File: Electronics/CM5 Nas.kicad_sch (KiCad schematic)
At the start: 0 parts

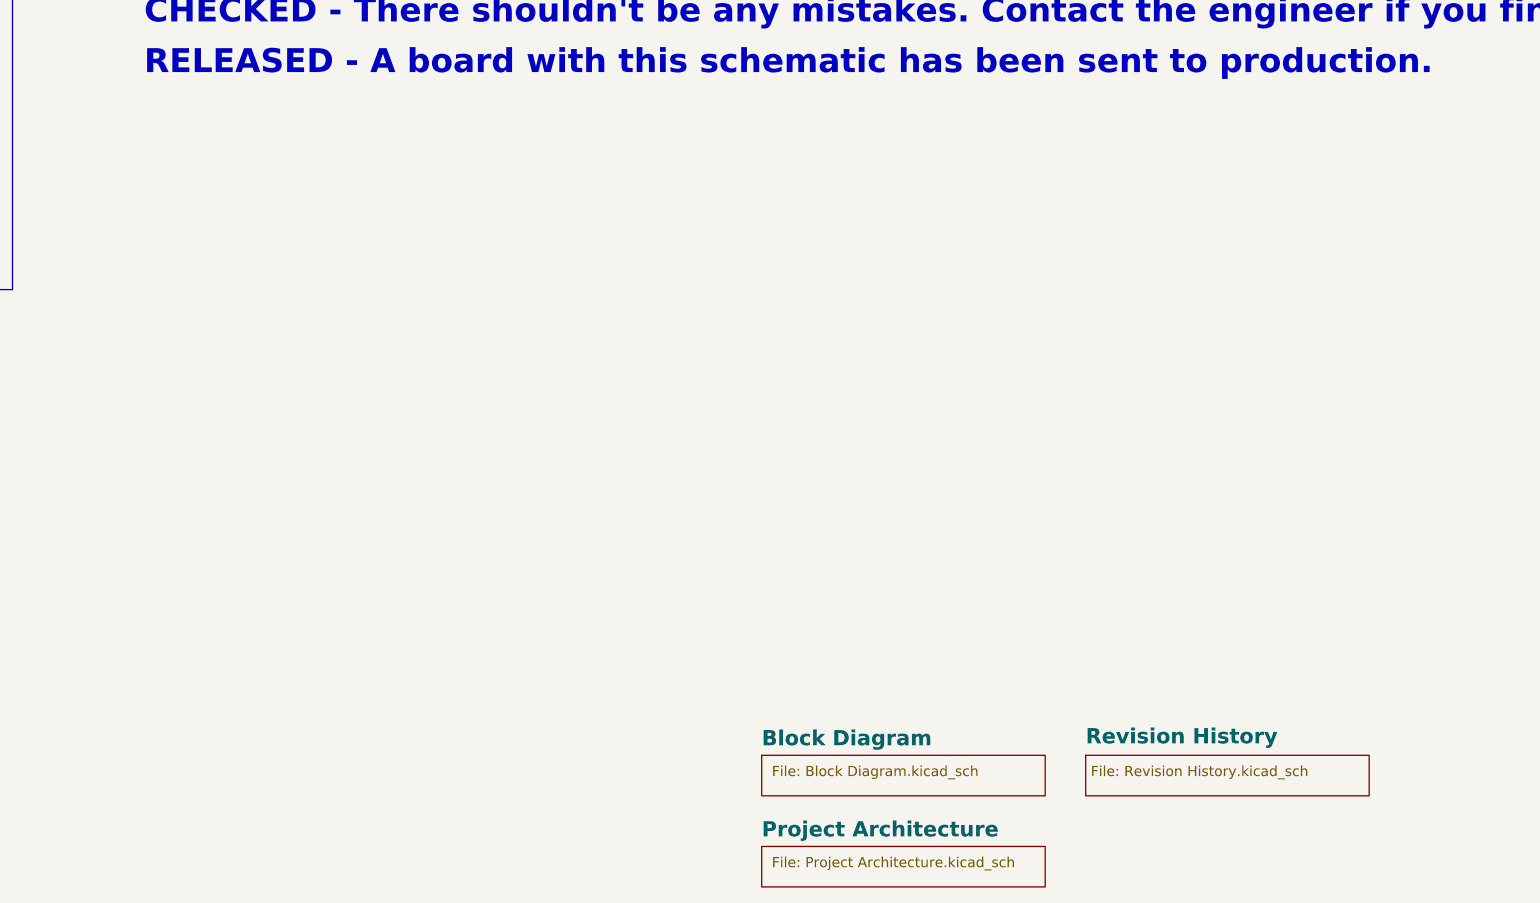
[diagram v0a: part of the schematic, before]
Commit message: Footprints selected, Hiracicle connections created, Pcb next
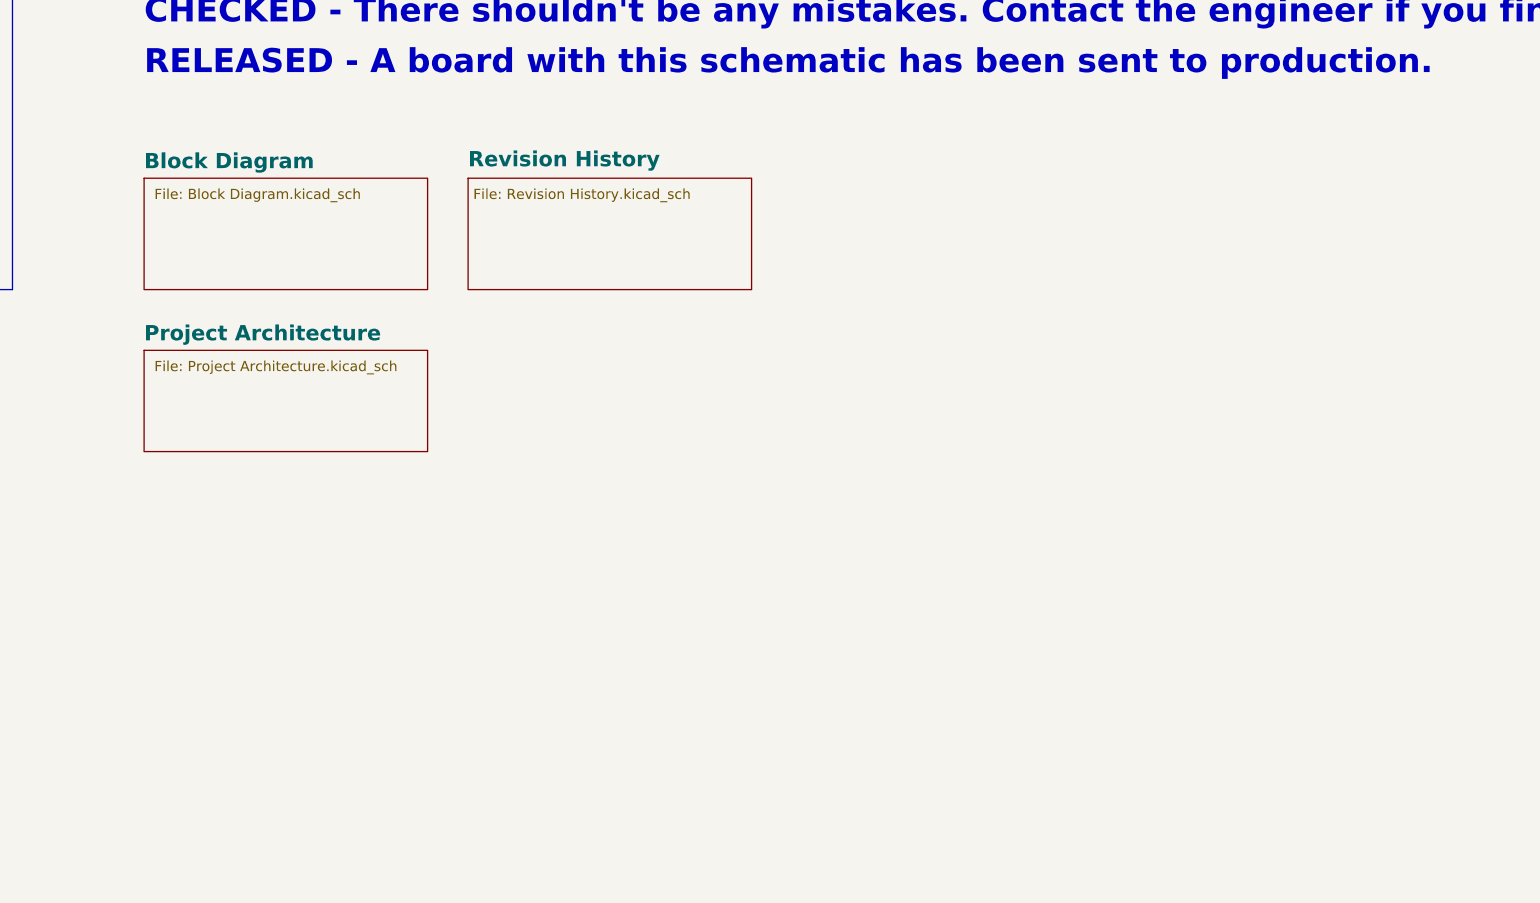
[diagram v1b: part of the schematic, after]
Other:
- company: ${COMPANY} -> (none)
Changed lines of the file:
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@@
 		(date "Last Modified Date")
 		(rev "${REVISION}")
-		(company "${COMPANY}")
 	)
 	(text "9"
@@
 	)
 	(sheet
-		(at 299.72 302.26)
-		(size 35.56 5.08)
+		(at 222.25 229.87)
+		(size 35.56 13.97)
 		(exclude_from_sim no)
 		(in_bom yes)
@@
 		)
 		(property "Sheetname" "Block Diagram"
-			(at 299.72 301.2309 0)
+			(at 222.25 228.8409 0)
 			(effects
 				(font
@@
 		)
 		(property "Sheetfile" "Block Diagram.kicad_sch"
-			(at 300.99 303.53 0)
+			(at 223.52 231.14 0)
 			(effects
 				(font
@@
 	)
 	(sheet
-		(at 340.36 302.26)
-		(size 35.56 5.08)
+		(at 262.89 229.87)
+		(size 35.56 13.97)
 		(exclude_from_sim no)
 		(in_bom yes)
@@
 		)
 		(property "Sheetname" "Revision History"
-			(at 340.36 300.99 0)
+			(at 262.89 228.6 0)
 			(effects
 				(font
@@
 		)
 		(property "Sheetfile" "Revision History.kicad_sch"
-			(at 340.995 303.53 0)
+			(at 263.525 231.14 0)
 			(effects
 				(font
@@
 	)
 	(sheet
-		(at 299.72 313.69)
-		(size 35.56 5.08)
+		(at 222.25 251.46)
+		(size 35.56 12.7)
 		(exclude_from_sim no)
 		(in_bom yes)
@@
 		)
 		(property "Sheetname" "Project Architecture"
-			(at 299.72 312.6609 0)
+			(at 222.25 250.4309 0)
 			(effects
 				(font
@@
 		)
 		(property "Sheetfile" "Project Architecture.kicad_sch"
-			(at 300.99 314.96 0)
+			(at 223.52 252.73 0)
 			(effects
 				(font
